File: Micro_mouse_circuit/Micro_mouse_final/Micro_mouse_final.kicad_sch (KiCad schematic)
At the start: 49 parts, among them J1 Conn_02x16_Odd_Even, J2 USB_C_Receptacle_PowerOnly_6P, J3 Conn_01x02, U1 HUSB237-AA001-DN06R, U10 AMS1117-3.3, U11 TPS22917DBV, U12 TPS22917DBV, U2 SK22D15L5, U3 LM2596SX-5_0/NOPB, U4 TP4056_C382139, U5 SN74LVC1G3157DCKR, U6 INA219AxDCN, U7 MT3608, U8 L298N_C19922, U9 L298N_C19922

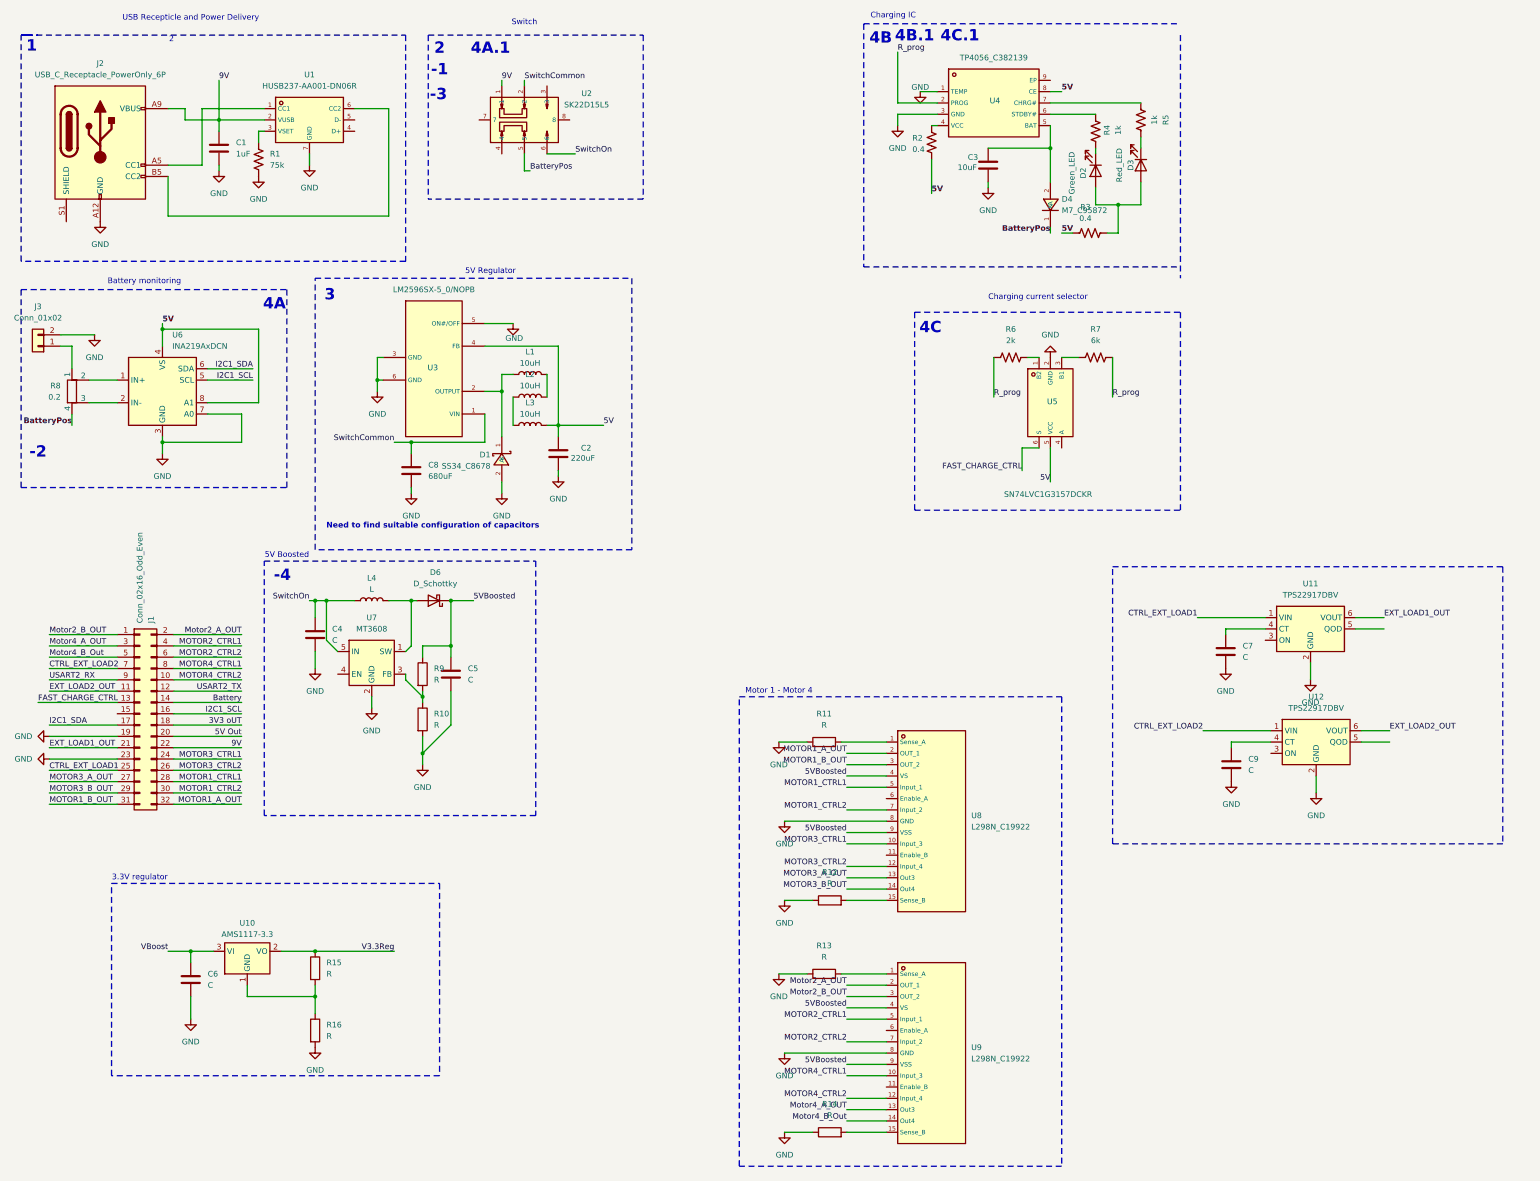
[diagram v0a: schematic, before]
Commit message: 02/28 submission
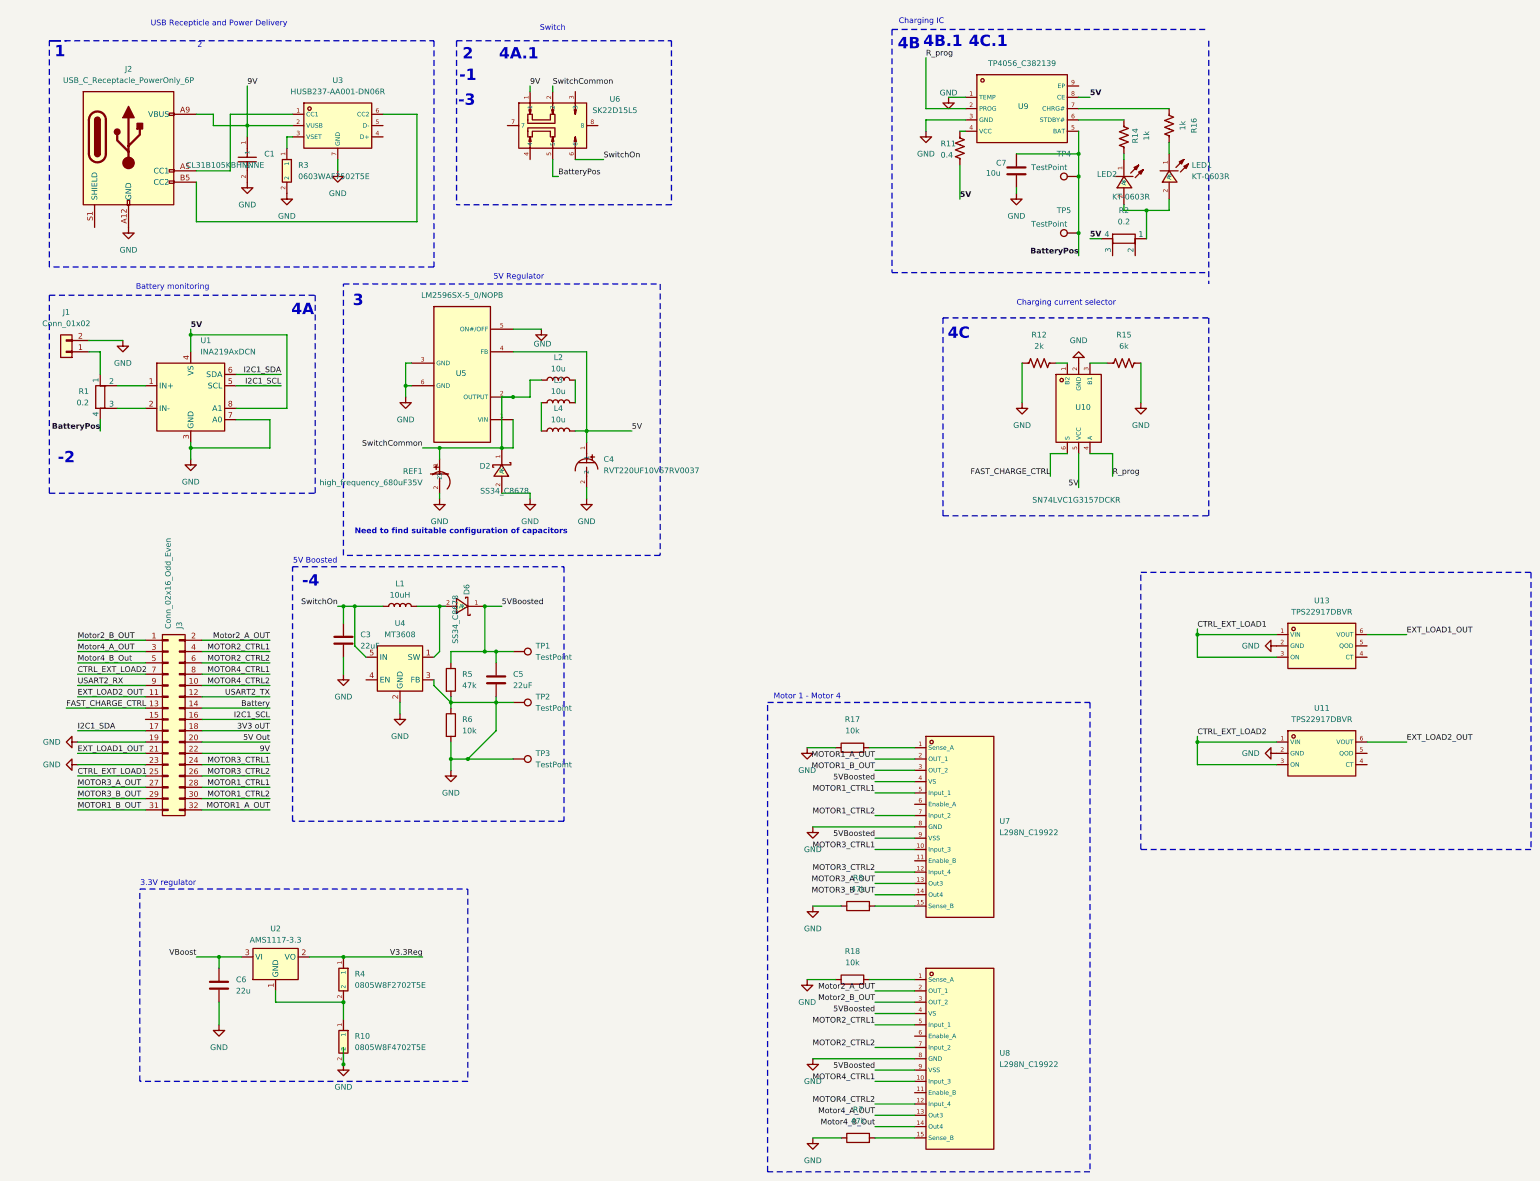
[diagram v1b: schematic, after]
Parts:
- removed C1: 1uF, symbol Device:C
- removed C2: 220uF, symbol Device:C
- removed C4, C9: C, symbol Device:C
- removed C8: 680uF, symbol Device:C
- removed D1: SS34_C8678, xxcustom_footprint:SMA_L4.3-W2.6-LS5.2-RD, symbol SS34_C8678:SS34_C8678
- removed D2: Green_LED, symbol Device:LED
- removed D3: Red_LED, symbol Device:LED
- removed D4: M7_C95872, footprint:SMA_L4.3-W2.6-LS5.2-RD, symbol M7_C95872:M7_C95872
- removed D6: D_Schottky, symbol Device:D_Schottky
- removed J1: Conn_02x16_Odd_Even, Connector_PinHeader_2.54mm:PinHeader_2x16_P2.54mm_Vertical, symbol Connector_Generic:Conn_02x16_Odd_Even
- removed J3: Conn_01x02, Connector_JST:JST_PH_S2B-PH-K_1x02_P2.00mm_Horizontal, symbol Connector_Generic:Conn_01x02
- removed R1: 75k, symbol Device:R_US
- removed R10, R11, R12, R13, R14, R15, R16, R9: R, symbol Device:R
- removed R2: 0.4, xxcustom_footprint:R0402, symbol Device:R_US
- removed R3: 0.4, symbol Device:R_US
- removed R4, R5: 1k, xxcustom_footprint:R0402, symbol Device:R_US
- removed R6: 2k, xxcustom_footprint:R0402, symbol Device:R_US
- removed R7: 6k, xxcustom_footprint:R0402, symbol Device:R_US
- removed R8: 0.2, xxcustom_footprint:R2512, symbol Device:R_Shunt
- removed U1: HUSB237-AA001-DN06R, xxcustom_footprint:TDFN-6_L2.0-W2.0-P0.65-TL-EP, symbol HUSB237-AA001-DN06R:HUSB237-AA001-DN06R
- removed U10: AMS1117-3.3, Package_TO_SOT_SMD:SOT-223-3_TabPin2, symbol Regulator_Linear:AMS1117-3.3
- removed U11, U12: TPS22917DBV, Package_TO_SOT_SMD:SOT-23-6, symbol Power_Management:TPS22917DBV
- removed U2: SK22D15L5, xxcustom_footprint:SW-TH_XKB_SK22D15L7, symbol SK22D15L5:SK22D15L5
- removed U3: LM2596SX-5_0/NOPB, xxcustom_footprint:TO-263-5_L10.2-W8.9-P1.70-TL, symbol LM2596SX-5_0/NOPB:LM2596SX-5_0/NOPB
- removed U4: TP4056_C382139, xxcustom_footprint:ESOP-8_L4.9-W3.9-P1.27-LS6.0-BL-EP, symbol TP4056_C382139:TP4056_C382139
- removed U5: SN74LVC1G3157DCKR, xxcustom_footprint:SC-70-6_L2.2-W1.3-P0.65-LS2.1-BR, symbol SN74LVC1G3157DCKR:SN74LVC1G3157DCKR
- removed U6: INA219AxDCN, Package_TO_SOT_SMD:SOT-23-8, symbol Sensor_Energy:INA219AxDCN
- removed U7: MT3608, Package_TO_SOT_SMD:SOT-23-6, symbol Regulator_Switching:MT3608
- removed U9: L298N_C19922, footprint:MULTIWATT-15_L19.6-W5.0-P1.27-L, symbol L298N_C19922:L298N_C19922
- added C1: CL31B105KBHNNNE, xxcustom_footprint:C1206, symbol CL31B105KBHNNNE:CL31B105KBHNNNE
- added C4: RVT220UF10V67RV0037, xxcustom_footprint:CAP-SMD_BD6.3-L6.6-W6.6-FD, symbol RVT220UF10V67RV0037:RVT220UF10V67RV0037
- added D2, D6: SS34_C8678, xxcustom_footprint:SMA_L4.3-W2.6-LS5.2-RD, symbol SS34_C8678:SS34_C8678
- added J1: Conn_01x02, Connector_JST:JST_PH_S2B-PH-K_1x02_P2.00mm_Horizontal, symbol Connector_Generic:Conn_01x02
- added J3: Conn_02x16_Odd_Even, Connector_PinHeader_2.54mm:PinHeader_2x16_P2.54mm_Vertical, symbol Connector_Generic:Conn_02x16_Odd_Even
- added LED1, LED2: KT-0603R, xxcustom_footprint:R0603, symbol KT-0603R:KT-0603R
- added R1, R2: 0.2, xxcustom_footprint:R2512, symbol Device:R_Shunt
- added R10: 0805W8F4702T5E, xxcustom_footprint:R0805, symbol 0805W8F4702T5E:0805W8F4702T5E
- added R11: 0.4, xxcustom_footprint:R0402, symbol Device:R_US
- added R12: 2k, xxcustom_footprint:C1206, symbol Device:R_US
- added R14, R16: 1k, xxcustom_footprint:R0402, symbol Device:R_US
- added R15: 6k, xxcustom_footprint:R0805, symbol Device:R_US
- added R17, R18, R6: 10k, xxcustom_footprint:C1206, symbol Device:R
- added R3: 0603WAF7502T5E, xxcustom_footprint:R0603, symbol 0603WAF7502T5E:0603WAF7502T5E
- added R4: 0805W8F2702T5E, xxcustom_footprint:R0805, symbol 0805W8F2702T5E:0805W8F2702T5E
- added R5, R7, R8: 47k, xxcustom_footprint:R0805, symbol Device:R
- added REF1: high_frequency_680uF35V, xxcustom_footprint:CAP-TH_BD10.0-P5.00-D1.0-FD, symbol high_frequency_680uF35V:high_frequency_680uF35V
- added TP1, TP2, TP3, TP4, TP5: TestPoint, TestPoint:TestPoint_Pad_2.5x2.5mm, symbol Connector:TestPoint
- added U1: INA219AxDCN, Package_TO_SOT_SMD:SOT-23-8, symbol Sensor_Energy:INA219AxDCN
- added U10: SN74LVC1G3157DCKR, xxcustom_footprint:SC-70-6_L2.2-W1.3-P0.65-LS2.1-BR, symbol SN74LVC1G3157DCKR:SN74LVC1G3157DCKR
- added U11, U13: TPS22917DBVR, xxcustom_footprint:SOT-23-6_L2.9-W1.6-P0.95-LS2.8-BR, symbol TPS22917DBVR:TPS22917DBVR
- added U2: AMS1117-3.3, Package_TO_SOT_SMD:SOT-223-3_TabPin2, symbol Regulator_Linear:AMS1117-3.3
- added U3: HUSB237-AA001-DN06R, xxcustom_footprint:TDFN-6_L2.0-W2.0-P0.65-TL-EP, symbol HUSB237-AA001-DN06R:HUSB237-AA001-DN06R
- added U4: MT3608, xxcustom_footprint:SOT-23-6_L2.9-W1.6-P0.95-LS2.8-BL, symbol Regulator_Switching:MT3608
- added U5: LM2596SX-5_0/NOPB, xxcustom_footprint:TO-263-5_L10.2-W8.9-P1.70-TL, symbol LM2596SX-5_0/NOPB:LM2596SX-5_0/NOPB
- added U6: SK22D15L5, xxcustom_footprint:SW-TH_XKB_SK22D15L7, symbol SK22D15L5:SK22D15L5
- added U7: L298N_C19922, xxcustom_footprint:MULTIWATT-15_L19.6-W5.0-P1.27-L, symbol L298N_C19922:L298N_C19922
- added U9: TP4056_C382139, xxcustom_footprint:ESOP-8_L4.9-W3.9-P1.27-LS6.0-BL-EP, symbol TP4056_C382139:TP4056_C382139
- C3: value 10uF -> 22uF; footprint (none) -> xxcustom_footprint:C1206
- C5: value C -> 22uF; footprint (none) -> xxcustom_footprint:C1206
- C6: value C -> 22u; footprint (none) -> xxcustom_footprint:C1206
- C7: value C -> 10u; footprint (none) -> xxcustom_footprint:CAP-SMD_L3.2-W1.6-RD-C7171
- J2: footprint (none) -> xxcustom_footprint:TYPE-C-SMD_TYPE-C-6P
- L2, L3: value 10uH -> 10u
- L4: value L -> 10u; footprint (none) -> xxcustom_footprint:L0805
- U8: footprint footprint:MULTIWATT-15_L19.6-W5.0-P1.27-L -> xxcustom_footprint:MULTIWATT-15_L19.6-W5.0-P1.27-L
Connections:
- net 3V3 oUT: now also J3.18 (Pin_18)
- net 5V: now also L4.2, C4.1, R11.1, R2.4, U1.4 (VS), U1.8 (A1), U10.5 (VCC), U5.4 (FB), U9.8 (CE); no longer L3.2
- net 5V Out: now also J3.20 (Pin_20)
- net 5VBoosted: now also D6.1 (K), R5.1, TP1.1, U7.4 (VS), U7.9 (VSS)
- net 9V: now also C1.1, J3.22 (Pin_22), U3.2 (VUSB), U6.1
- net Battery: now also J3.14 (Pin_14)
- net BatteryPos: now also C7.1, R1.4, TP4.1, TP5.1, U6.5, U9.5 (BAT)
- net CTRL_EXT_LOAD1: now also J3.25 (Pin_25), U13.1 (VIN), U13.3 (ON)
- net CTRL_EXT_LOAD2: now also J3.7 (Pin_7), U11.1 (VIN), U11.3 (ON)
- net EXT_LOAD1_OUT: now also J3.21 (Pin_21), U13.6 (VOUT)
- net EXT_LOAD2_OUT: now also J3.11 (Pin_11), U11.6 (VOUT)
- net FAST_CHARGE_CTRL: now also J3.13 (Pin_13), U10.6 (S)
- net GND: now also C1.2, C4.2, D2.2 (A), J1.2 (Pin_2), J3.19 (Pin_19), J3.23 (Pin_23), R10.2, R12.1, R15.1, R17.1, R18.1, R3.2, R5.2, R6.1, R6.2, R7.1, R8.1, REF1.2, TP2.1, TP3.1, U1.3 (GND), U1.7 (A0), U10.2 (GND), U11.2 (GND), U13.2 (GND), U3.7 (GND), U4.2 (GND), U4.3 (FB), U5.3 (GND), U5.5 (ON#/OFF), U5.6 (GND), U7.8 (GND), U9.1 (TEMP), U9.3 (GND)
- net I2C1_SCL: now also J3.16 (Pin_16), U1.5 (SCL)
- net I2C1_SDA: now also J3.17 (Pin_17), U1.6 (SDA)
- net MOTOR1_A_OUT: now also J3.32 (Pin_32), U7.2 (OUT_1); no longer U8.2 (OUT_1)
- net MOTOR1_B_OUT: now also J3.31 (Pin_31), U7.3 (OUT_2); no longer U8.3 (OUT_2)
- net MOTOR1_CTRL1: now also J3.28 (Pin_28), U7.5 (Input_1); no longer U8.5 (Input_1)
- net MOTOR1_CTRL2: now also J3.30 (Pin_30), U7.7 (Input_2); no longer U8.7 (Input_2)
- net MOTOR2_CTRL1: now also U8.5 (Input_1), J3.4 (Pin_4)
- net MOTOR2_CTRL2: now also U8.7 (Input_2), J3.6 (Pin_6)
- net MOTOR3_A_OUT: now also J3.27 (Pin_27), U7.13 (Out3); no longer U8.13 (Out3)
- net MOTOR3_B_OUT: now also J3.29 (Pin_29), U7.14 (Out4); no longer U8.14 (Out4)
- net MOTOR3_CTRL1: now also J3.24 (Pin_24), U7.10 (Input_3); no longer U8.10 (Input_3)
- net MOTOR3_CTRL2: now also J3.26 (Pin_26), U7.12 (Input_4); no longer U8.12 (Input_4)
- net MOTOR4_CTRL1: now also U8.10 (Input_3), J3.8 (Pin_8)
- net MOTOR4_CTRL2: now also U8.12 (Input_4), J3.10 (Pin_10)
- net Motor2_A_OUT: now also U8.2 (OUT_1), J3.2 (Pin_2)
- net Motor2_B_OUT: now also U8.3 (OUT_2), J3.1 (Pin_1)
- net Motor4_A_OUT: now also U8.13 (Out3), J3.3 (Pin_3)
- net Motor4_B_Out: now also U8.14 (Out4), J3.5 (Pin_5)
- net R_prog: now also U10.4 (A), U9.2 (PROG)
- net SwitchCommon: now also L2.1, D2.1 (K), REF1.1, U5.1 (VIN), U5.2 (OUTPUT), U6.2
- net SwitchOn: now also C3.1, L1.1, U4.5 (IN), U6.6; no longer L4.1
- net USART2_RX: now also J3.9 (Pin_9)
- net USART2_TX: now also J3.12 (Pin_12)
- net V3.3Reg: now also R4.1, U2.2 (VO)
- net VBoost: now also U2.3 (VI)
- net at L3.1: now also L4.1; no longer L2.1
- net at L1.2: now also D6.2 (A), U4.1 (SW); no longer L2.2
- net at J2.A5 (CC1): now also U3.1 (CC1)
- net at J2.B5 (CC2): now also U3.6 (CC2)
- net at U8.1 (Sense_A): now also R18.2
- net at U8.15 (Sense_B): now also R7.2
- new net: R3.1, U3.3 (VSET)
- new net: R17.2, U7.1 (Sense_A)
- new net: R14.1, U9.6 (STDBY#)
- new net: LED2.1 (K), R14.2
- new net: R15.2, U10.3 (B1)
- new net: R11.2, U9.4 (VCC)
- new net: R16.2, U9.7 (CHRG#)
- new net: R1.2, U1.1 (IN+)
- new net: R1.3, U1.2 (IN-)
- new net: LED1.1 (K), R16.1
- new net: LED1.2 (A), LED2.2 (A), R2.1
- new net: R10.1, R4.2, U2.1 (GND)
- new net: L2.2, L3.2
- new net: R12.2, U10.1 (B2)
- new net: R8.2, U7.15 (Sense_B)
- new net: J1.1 (Pin_1), R1.1
